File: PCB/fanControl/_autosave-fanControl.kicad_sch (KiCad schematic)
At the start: 105 parts, among them J1 USB_B_Micro, J2 Barrel_Jack_Switch, J3 Conn_01x03, J4 Conn_01x06, J5 Conn_01x04, Q1 FDD4243, Q2 BSS84, Q3 BC547, Q4 BC847B, Q5 BC847B, Q6 BRCS4484, Q7 BC847B, Q8 BSS84, Q9 BC847B, U1 DS18B20, U2 CH340B, U3 LM2575BT-ADJ, U4 LM1117, U5 ESP-12E, Y1 12M

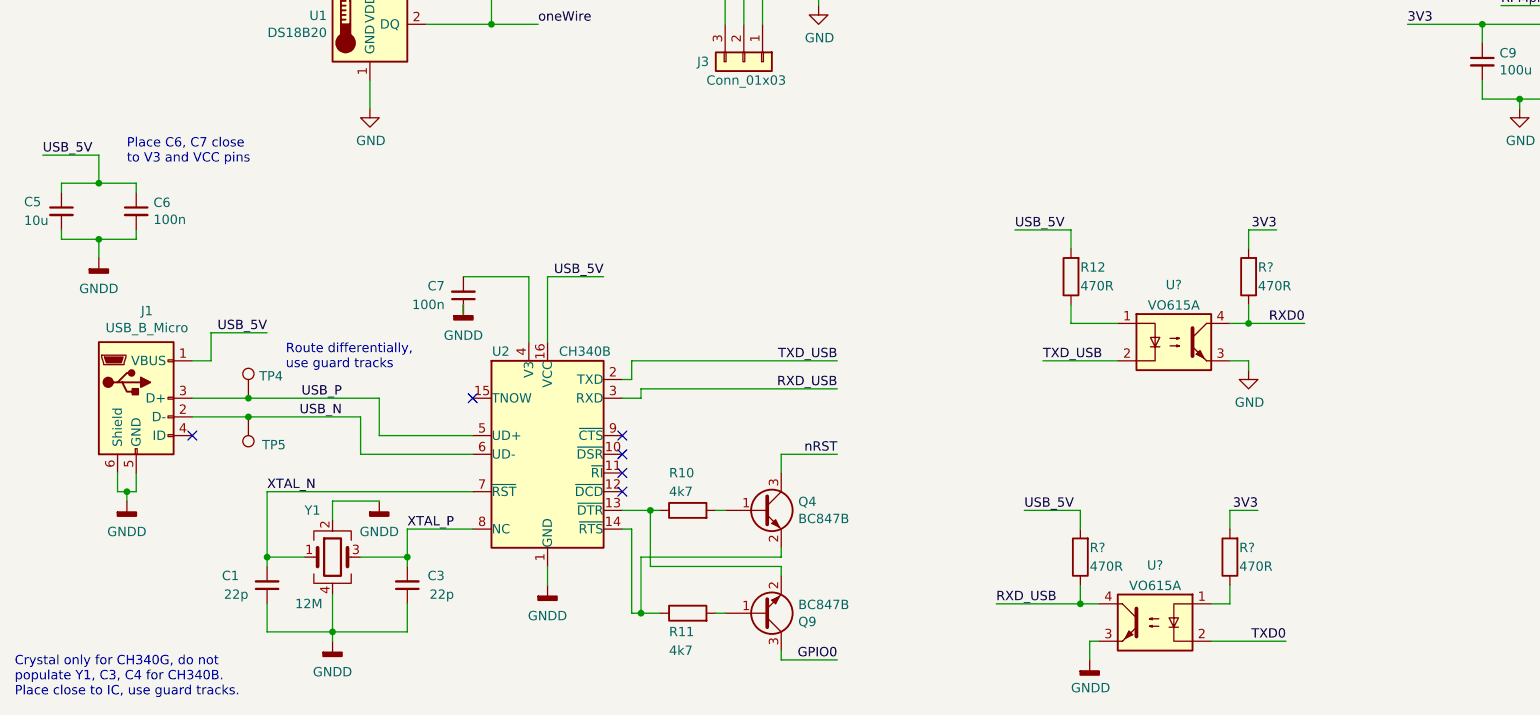
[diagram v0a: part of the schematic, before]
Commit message: before optocouplers
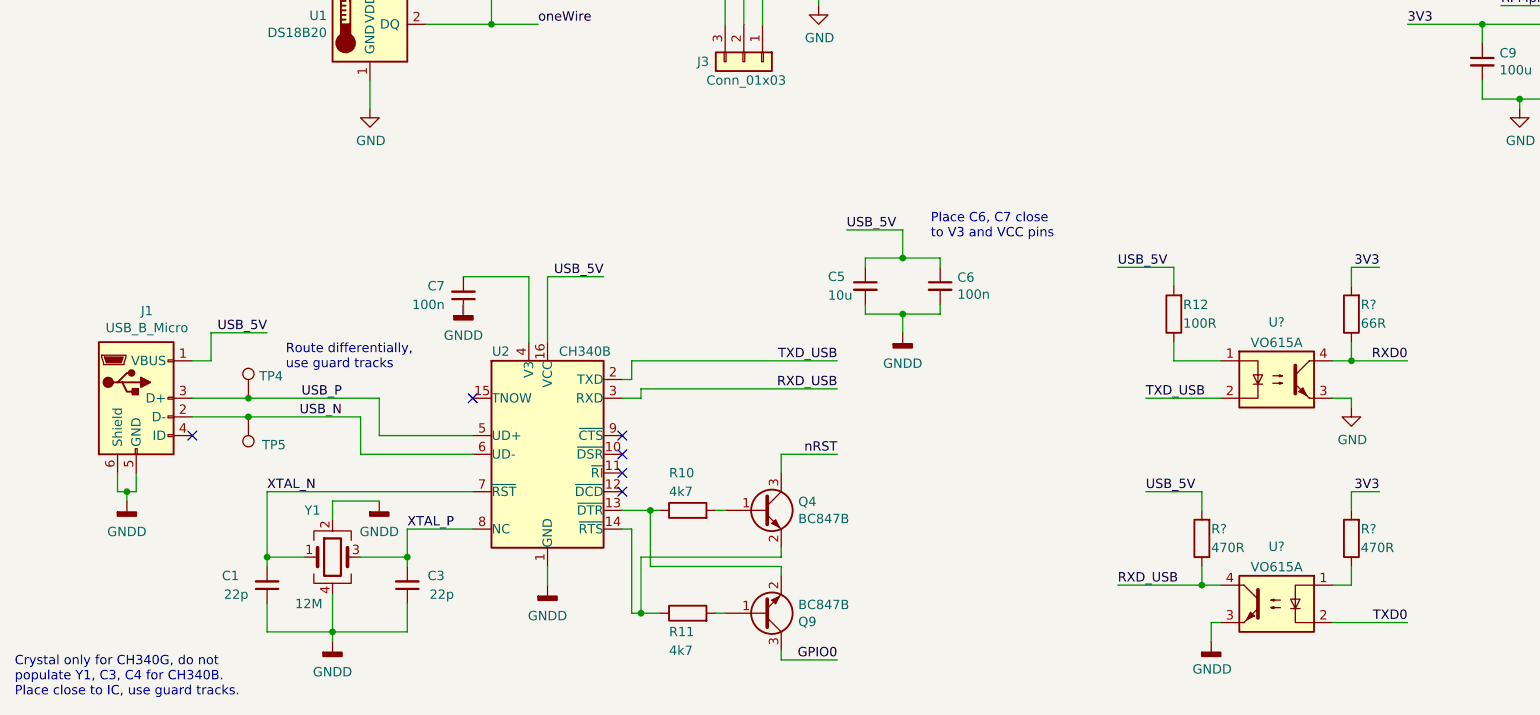
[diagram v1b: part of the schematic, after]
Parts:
- removed R?: 470R, agro-footprint:RES_0805, symbol Device:R
- added R?: 470R, agro-footprint:RES_0805, symbol Device:R
- R12: value 470R -> 100R; LCSC C114747 -> (none)
- R?: value 470R -> 66R; LCSC C114747 -> (none)
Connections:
- net 3V3: now also R?.2
- net at U?.1: now also R?.1
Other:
- moved on the sheet: C5, C6, R12, R?, U?
